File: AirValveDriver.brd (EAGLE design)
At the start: 71.1 x 62.2 mm, 16 parts, among them IC2 NE555, Q1 2N2222, Q2 STF40NF06

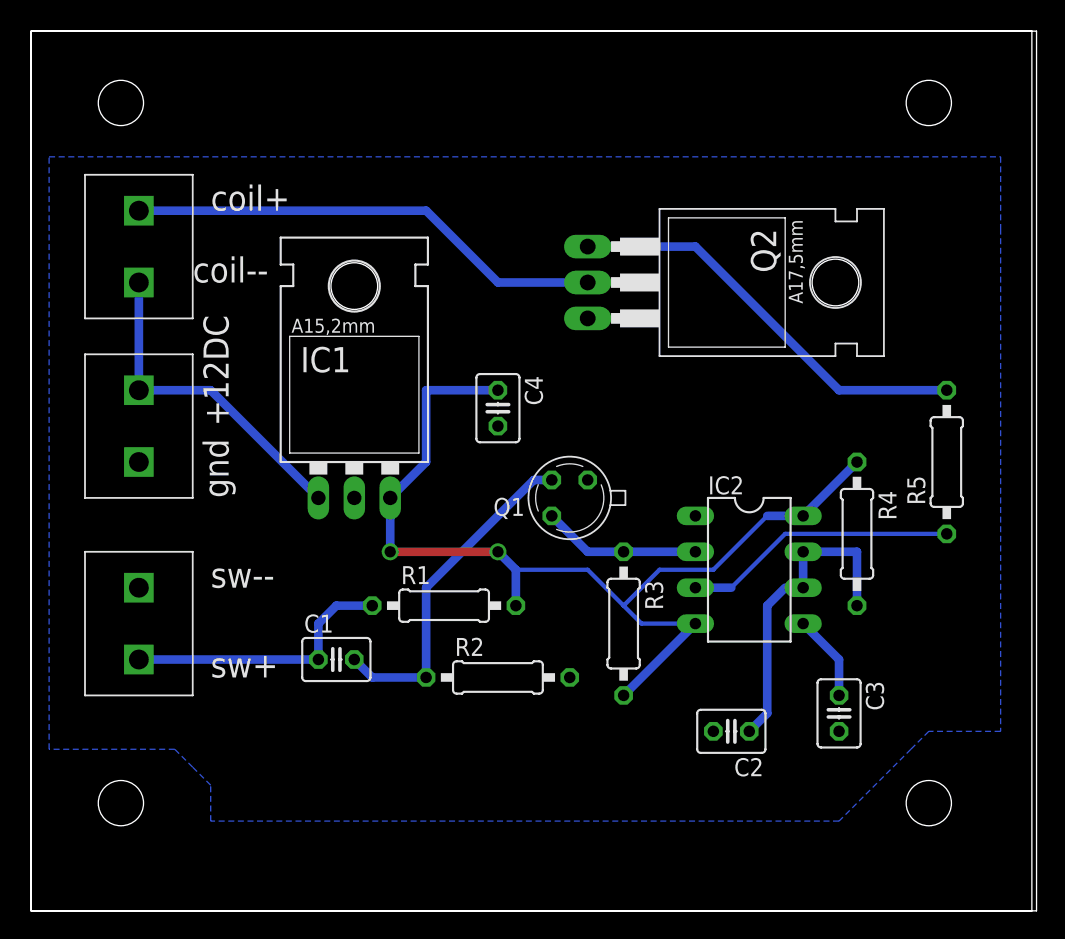
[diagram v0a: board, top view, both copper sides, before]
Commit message: updated after DRC
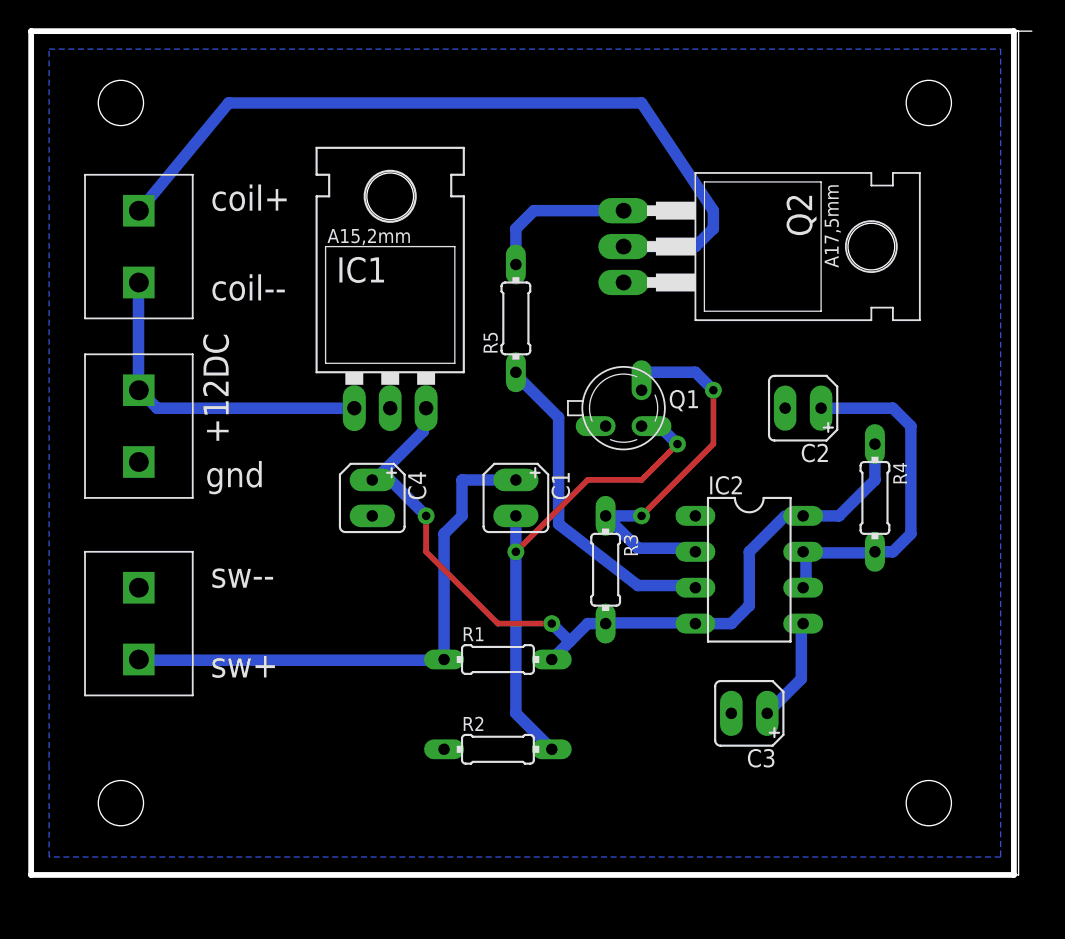
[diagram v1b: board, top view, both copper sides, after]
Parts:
- added DRILEGEND: (no value), drilegend:DRILEGEND
- C1: device resistor:C025-030X050 -> myDevices:CPOL_PKG
- C2, C4: value 10u -> CAPACITOR_POLARIZED; device resistor:C025-030X050 -> myDevices:CPOL_PKG
- C3: value 0.1u -> CAPACITOR_POLARIZED; device resistor:C025-030X050 -> myDevices:CPOL_PKG
- IC1: value (none) -> LM7805
- Q1: device transistor-npn:TO18 -> myDevices:TO18
- R1, R2, R3, R4, R5: device resistor:0207/10 -> myDevices:RESISTOR_PKG
- moved R5 32.1 mm to (34.3, 55.9)
- moved C2 23.4 mm to (54.6, 49.5)
- moved C1 17.1 mm to (34.3, 43.2), turned to 270 degrees
- moved C4 10.9 mm to (24.1, 43.2)
- moved Q1 7.41 mm to (41.9, 49.5), turned to 0 degrees
- moved IC1 6.84 mm to (25.4, 53.3)
- moved C3 6.35 mm to (50.8, 27.9), turned to 180 degrees
- moved R1 5.39 mm to (33.0, 31.8)
- moved R2 5.08 mm to (33.0, 25.4)
- moved R3 4.02 mm to (40.6, 38.1)
- moved Q2 3.59 mm to (48.3, 61.0)
- moved R4 2.84 mm to (59.7, 43.2)
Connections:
- net +5V: now also C4.+; no longer C4.1
- net AGND: now also C2.-, C3.-, C4.-, R2.1; no longer C2.2, C3.2, C4.2, R2.2
- net N$1: now also C3.+; no longer C3.1
- net N$10: now also C2.+; no longer C2.1
- net N$5: now also C1.+; no longer C1.1
- net N$6: now also C1.-, R2.2; no longer C1.2, R2.1
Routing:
- net N$4: track 33.9 -> 57.1 mm
- net N$5: track 19.6 -> 39.3 mm
- net N$2: track 29.6 -> 12.0 mm
- net N$7: track 11.2 -> 27.9 mm, vias 0 -> 2
- net +5V: track 71.7 -> 59.7 mm
- net N$6: track 24.0 -> 35.2 mm, vias 0 -> 2
- net OUTPUT_1: track 19.4 -> 23.2 mm
- net N$10: track 22.6 -> 25.3 mm
- net N$1: track 6.13 -> 7.37 mm
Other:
- board size 71.1 x 62.2 mm -> 70.8 x 59.7 mm
- board text added: "01-16"
- board text added: "01-20"
- board text added: "LAYER-STACK"
